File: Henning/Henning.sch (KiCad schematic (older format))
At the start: 19 parts, among them P1 RS232, P2 EBUS, Q1 BD645, U1 4011, U2 CNY17-1, U3 78L05, U4 CNY17-1

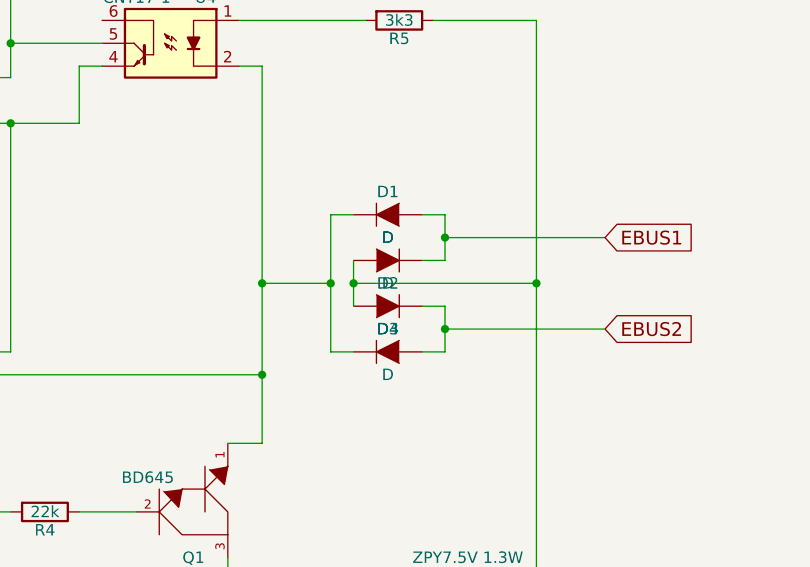
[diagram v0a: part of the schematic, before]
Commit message: Fixed PCB
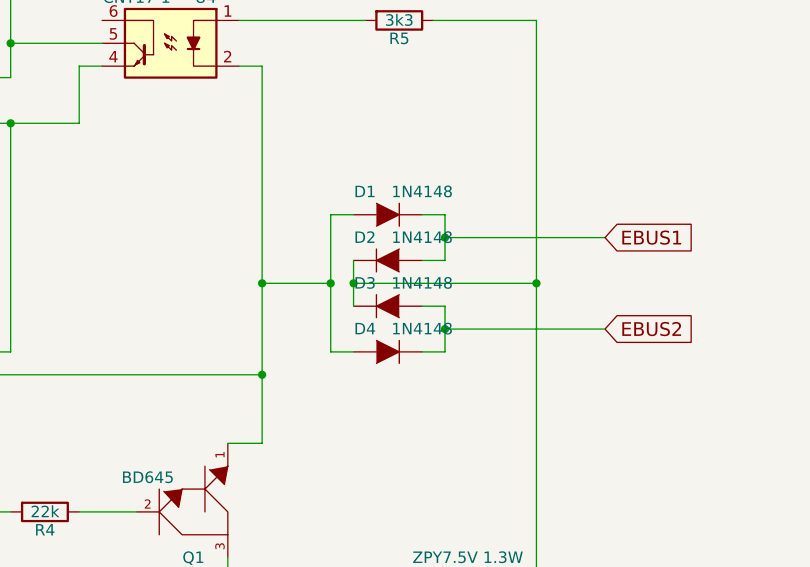
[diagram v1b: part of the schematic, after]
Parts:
- D1, D2, D3, D4: value D -> 1N4148
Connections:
- net EBUS1: now also D1.1 (K), D2.2 (A); no longer D1.2 (A), D2.1 (K)
- net EBUS2: now also D3.2 (A), D4.1 (K); no longer D3.1 (K), D4.2 (A)
- net at D5.1 (K), R5.1, U3.1 (VI): now also D2.1 (K), D3.1 (K); no longer D2.2 (A), D3.2 (A)
- net at C1.2, Q1.1, U3.2 (GND)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: now also D1.2 (A), D4.2 (A); no longer D1.1 (K), D4.1 (K)
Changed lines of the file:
@@
 U 1 1 57E456DB
 P 8750 2200
-F 0 "D1" H 8750 2300 50  0000 C CNN
-F 1 "D" H 8750 2100 50  0000 C CNN
+F 0 "D1" H 8850 2300 50  0000 C CNN
+F 1 "1N4148" H 8600 2300 50  0000 C CNN
 F 2 "Diodes_ThroughHole:Diode_DO-35_SOD27_Horizontal_RM10" H 8750 2200 50  0001 C CNN
 F 3 "" H 8750 2200 50  0000 C CNN
 	1    8750 2200
-	1    0    0    -1
+	-1   0    0    -1
 $EndComp
 $Comp
@@
 U 1 1 57E45729
 P 8750 2400
-F 0 "D2" H 8750 2500 50  0000 C CNN
-F 1 "D" H 8750 2300 50  0000 C CNN
+F 0 "D2" H 8650 2300 50  0000 C CNN
+F 1 "1N4148" H 8900 2300 50  0000 C CNN
 F 2 "Diodes_ThroughHole:Diode_DO-35_SOD27_Horizontal_RM10" H 8750 2400 50  0001 C CNN
 F 3 "" H 8750 2400 50  0000 C CNN
 	1    8750 2400
-	-1   0    0    1
+	1    0    0    1
 $EndComp
 $Comp
@@
 U 1 1 57E45775
 P 8750 2600
-F 0 "D3" H 8750 2700 50  0000 C CNN
-F 1 "D" H 8750 2500 50  0000 C CNN
+F 0 "D3" H 8650 2500 50  0000 C CNN
+F 1 "1N4148" H 8900 2500 50  0000 C CNN
 F 2 "Diodes_ThroughHole:Diode_DO-35_SOD27_Horizontal_RM10" H 8750 2600 50  0001 C CNN
 F 3 "" H 8750 2600 50  0000 C CNN
 	1    8750 2600
-	-1   0    0    1
+	1    0    0    1
 $EndComp
 $Comp
@@
 U 1 1 57E457DF
 P 8750 2800
-F 0 "D4" H 8750 2900 50  0000 C CNN
-F 1 "D" H 8750 2700 50  0000 C CNN
+F 0 "D4" H 8850 2900 50  0000 C CNN
+F 1 "1N4148" H 8600 2900 50  0000 C CNN
 F 2 "Diodes_ThroughHole:Diode_DO-35_SOD27_Horizontal_RM10" H 8750 2800 50  0001 C CNN
 F 3 "" H 8750 2800 50  0000 C CNN
 	1    8750 2800
-	1    0    0    -1
+	-1   0    0    -1
 $EndComp
 Wire Wire Line
